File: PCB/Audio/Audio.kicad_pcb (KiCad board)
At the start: 2 copper layers, 70 x 70 mm, 42 parts, among them J1 Battery, J3 TC2030-USB-NL-DS, J4 TF_PUSH, J5 USB-C-Socket-H, Q2 CJ2301, SW1 SW_Push, U1 R, U2 L, U3 TP4054, U4 ME6211C33M5G-N, U6 ESP32-S3-MINI-1

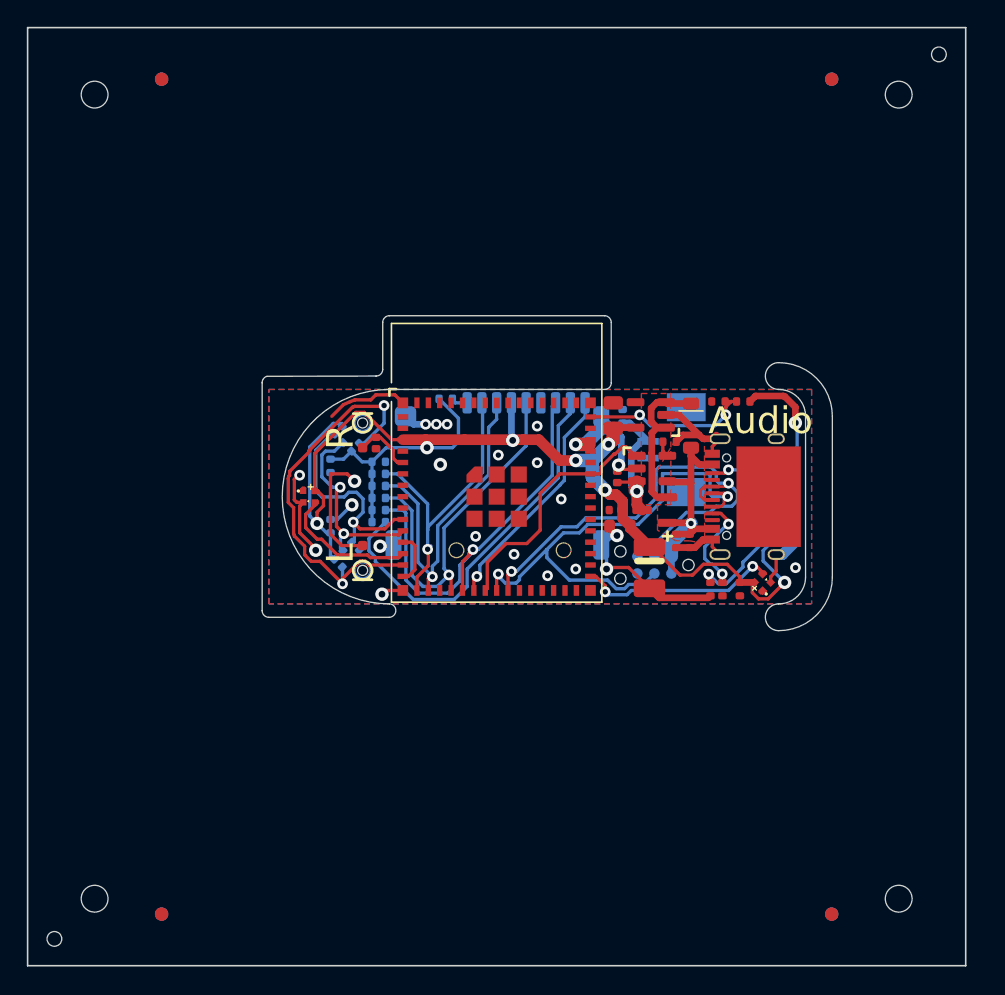
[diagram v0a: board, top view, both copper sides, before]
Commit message: New layout
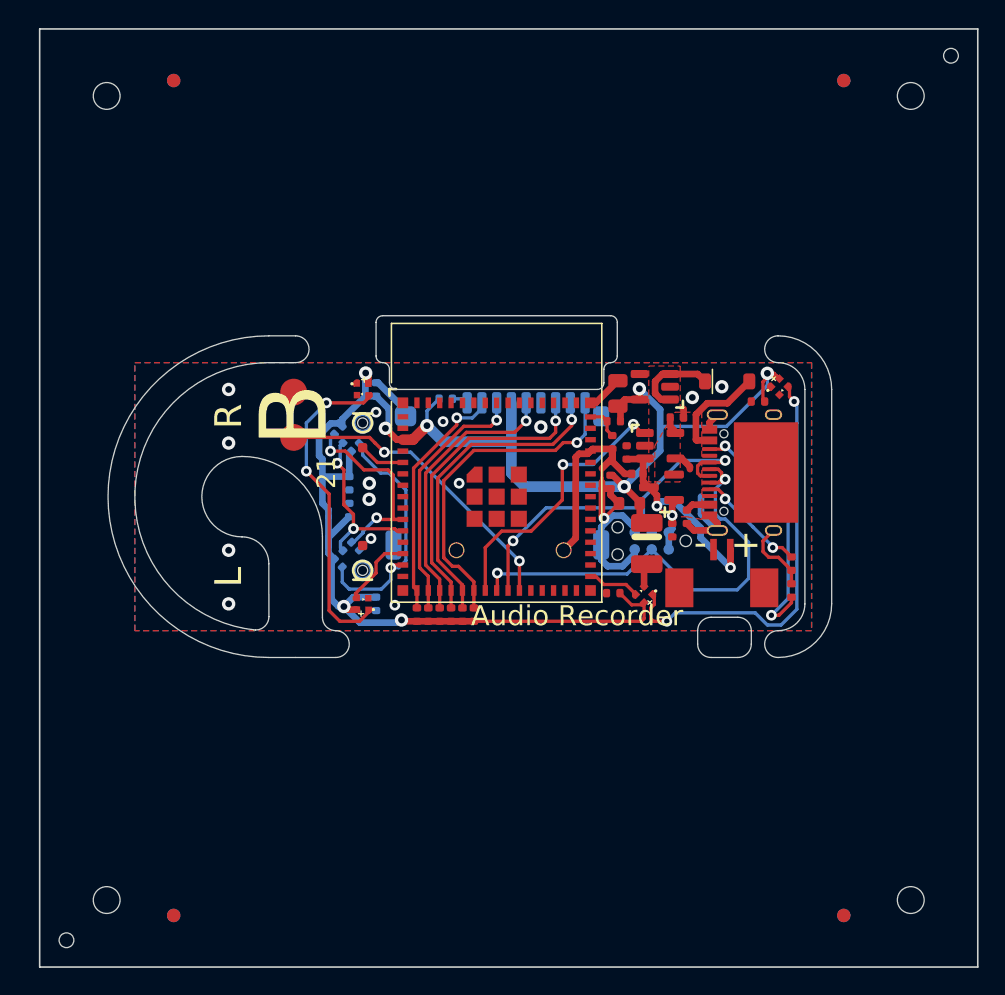
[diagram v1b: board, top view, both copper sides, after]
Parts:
- added C10: 100nF, RevK:C_0402, F.Cu at (119.5, 92.9)
- added C5: 100nF, RevK:C_0402, B.Cu at (91.0, 108.0)
- added D6: XL-1010RGBC-WS2812B, RevK:SMD1010, F.Cu at (121.1, 91.8)
- added J2: Reset, RevK:AA-Pad, F.Cu at (84.8, 93.9)
- added R3: 10K, RevK:R_0402, F.Cu at (98.3, 108.8)
- C7, J1, R10, R11, R12, R13, R9: moved to F.Cu
- D4: value ~ -> XL-1010RGBC-WS2812B; footprint RevK:DFN1006-2L -> RevK:SMD1010
- moved R13 10.9 mm to (94.0, 108.8), turned to 90 degrees
- moved R12 10.3 mm to (94.9, 108.8), turned to 90 degrees
- moved R11 9.82 mm to (95.8, 108.8), turned to 90 degrees
- moved R2 9.77 mm to (108.7, 94.4)
- moved J1 9.64 mm to (116.8, 105.1), turned to 180 degrees
- moved R10 9.49 mm to (96.6, 108.8), turned to 90 degrees
- moved C4 9.45 mm to (108.7, 107.2), turned to 180 degrees
- moved R9 9.31 mm to (97.5, 108.8), turned to 90 degrees
- moved D5 8.94 mm to (90.0, 108.0), turned to 180 degrees
- moved D1 8.89 mm to (111.0, 107.3), turned to -135 degrees
- moved C9 8.49 mm to (108.6, 95.9), turned to -90 degrees
- moved R6 6.05 mm to (122.0, 107.0), turned to -90 degrees
- moved R5 5.49 mm to (122.0, 105.0)
- moved C6 5.40 mm to (91.0, 92.0), turned to 90 degrees
- moved D3 4.26 mm to (117.2, 91.4), turned to 0 degrees
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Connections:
- D1 pad 1: unconnected-(D1-O-Pad1) -> Net-(D1-O)
- D4 pad 1: BUTTON -> unconnected-(D4-O-Pad1)
- D4 pad 2: GND -> +3V3
- D5 pad 1: unconnected-(D5-O-Pad1)_1 -> Net-(D4-I)
- J1 pad 1: GND -> VBAT
- J1 pad 2: VBAT -> GND
- J4 pad 8: Net-(J4-DAT1) -> SDDAT1
- R9 pad 2: Net-(J4-DAT1) -> SDDAT1
- U6 pad 12: GND -> unconnected-(U6-GPIO8-Pad12)
- U6 pad 15: GND -> unconnected-(U6-GPIO11-Pad15)
- U6 pad 18: unconnected-(U6-GPIO14-Pad18) -> SDSCK
- U6 pad 19: SDSCK -> SDMISO
- U6 pad 20: SDMISO -> SDDAT1
- U6 pad 25: unconnected-(U6-GPIO21-Pad25) -> Net-(J2-Pin_2)
- U6 pad 40: CHARGING -> unconnected-(U6-GPIO44-Pad40)
- U6 pad 6: GND -> unconnected-(U6-GPIO2-Pad6)
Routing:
- net Net-(D1-O): track 0.00 -> 30.9 mm, vias 0 -> 2
- net Net-(J4-DAT1): track 29.0 -> 0.00 mm
- net Net-(D4-I): track 0.00 -> 23.9 mm, vias 0 -> 2
- net SDDAT1: track 0.00 -> 23.7 mm, vias 0 -> 1
- net Net-(J2-Pin_2): track 0.00 -> 22.9 mm, vias 0 -> 2
- net GND: track 72.4 -> 54.6 mm, vias 23 -> 15
- net SCK: track 30.2 -> 19.0 mm, vias 2 -> 1
- net BLINK: track 14.7 -> 3.96 mm, vias 2 -> 0
- net Net-(U6-EN): track 12.8 -> 2.60 mm, vias 2 -> 0
- net D+: track 36.8 -> 28.4 mm
- net SDMISO: track 31.3 -> 23.3 mm
- net SDCD: track 17.4 -> 25.0 mm
- net SDSCK: track 27.4 -> 21.0 mm
- net SDMOSI: track 24.9 -> 19.1 mm
- net Net-(D3-K): track 11.8 -> 6.38 mm
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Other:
- board text added: "1"
- board text added: "12 13 15 16 17 6 7 10"
- board text added: "18"
- board text added: "21"
- board text added: "44"
- board text added: "9"
- board text added: "A"
- board text added: "Audio Recorder"
- board text added: "BTN"
- board text added: "CHG"
- board text added: "LED"
- board text added: "Made in China"
- board text added: "SS MOSI SCK MISO CD WS SD SCK"
- board text removed: "Audio"
